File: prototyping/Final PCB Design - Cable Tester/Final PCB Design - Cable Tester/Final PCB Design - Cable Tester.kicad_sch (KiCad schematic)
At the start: 43 parts, among them J1 USB_B_Micro, J17 Banana Jack, J2 UPDI, J20 SFML-110-02-L-D-A, J4 MEM2061-01-188-00-A_REVA, J5 Barrel Jack 9V, J6 Touchscreen HMI, Q1 2N3904, SW1 Rocker Switch, U1 AVR128DB64x-xMR, U2 LP2985-3.3, U3 LM7805_TO220, U4 FT232RL, U6 J104D2C5VDC.15S, U7 CD74HC4050M96

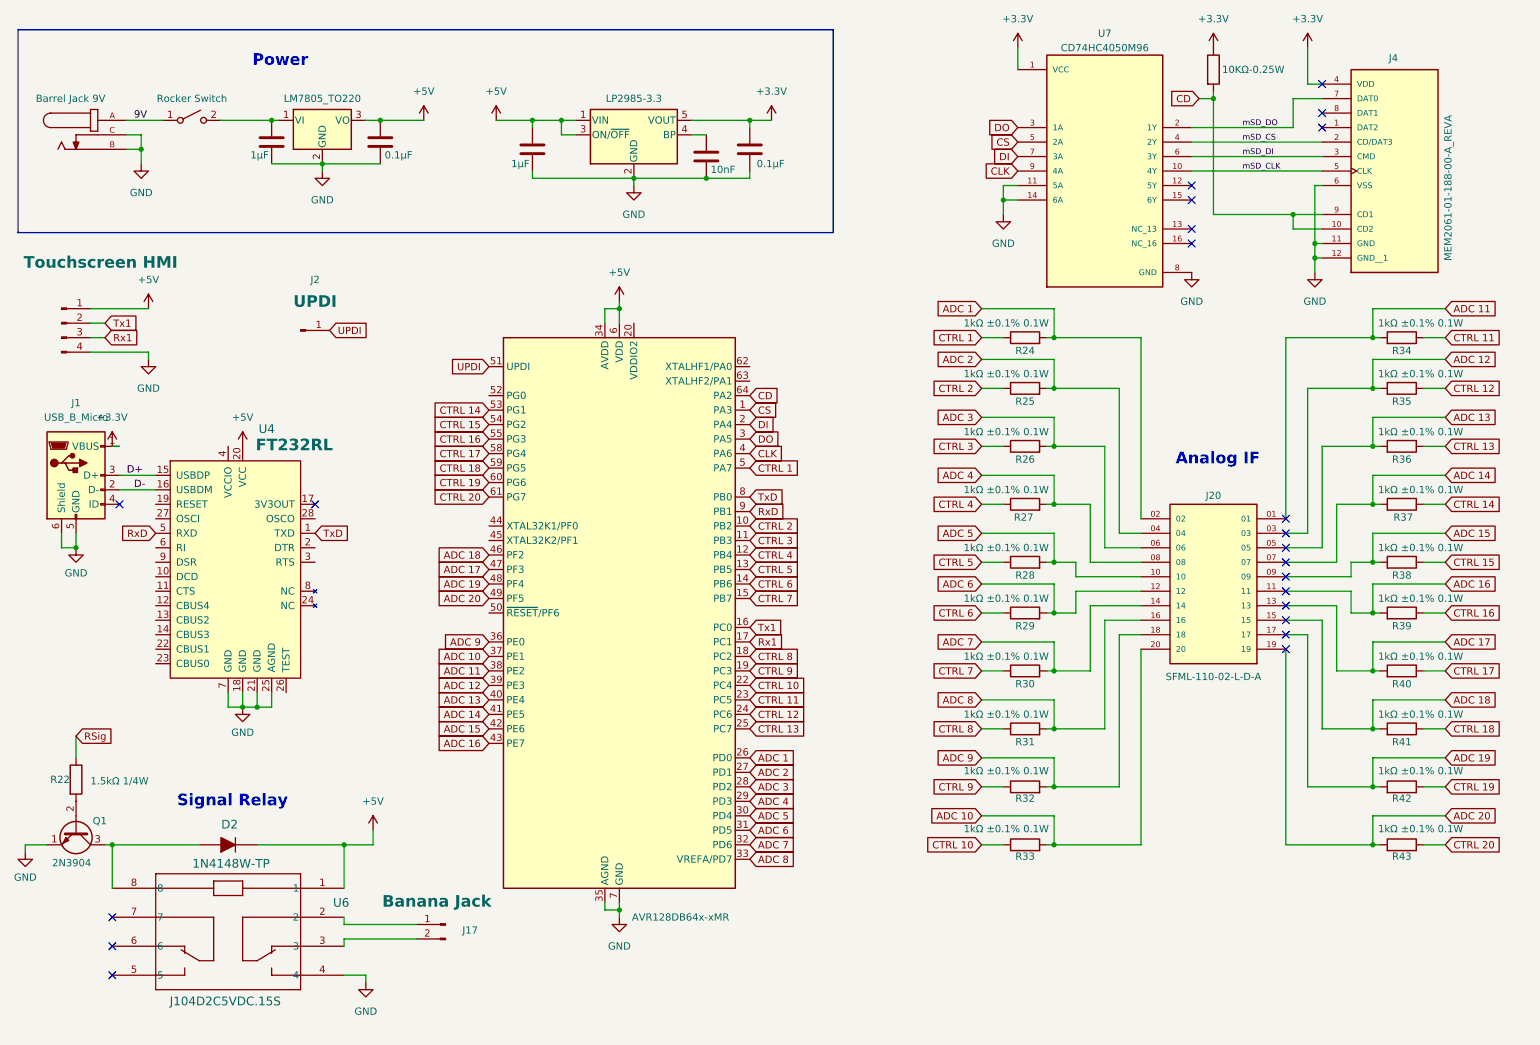
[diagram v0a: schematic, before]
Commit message: Final PCB Schematic and PCB layout update
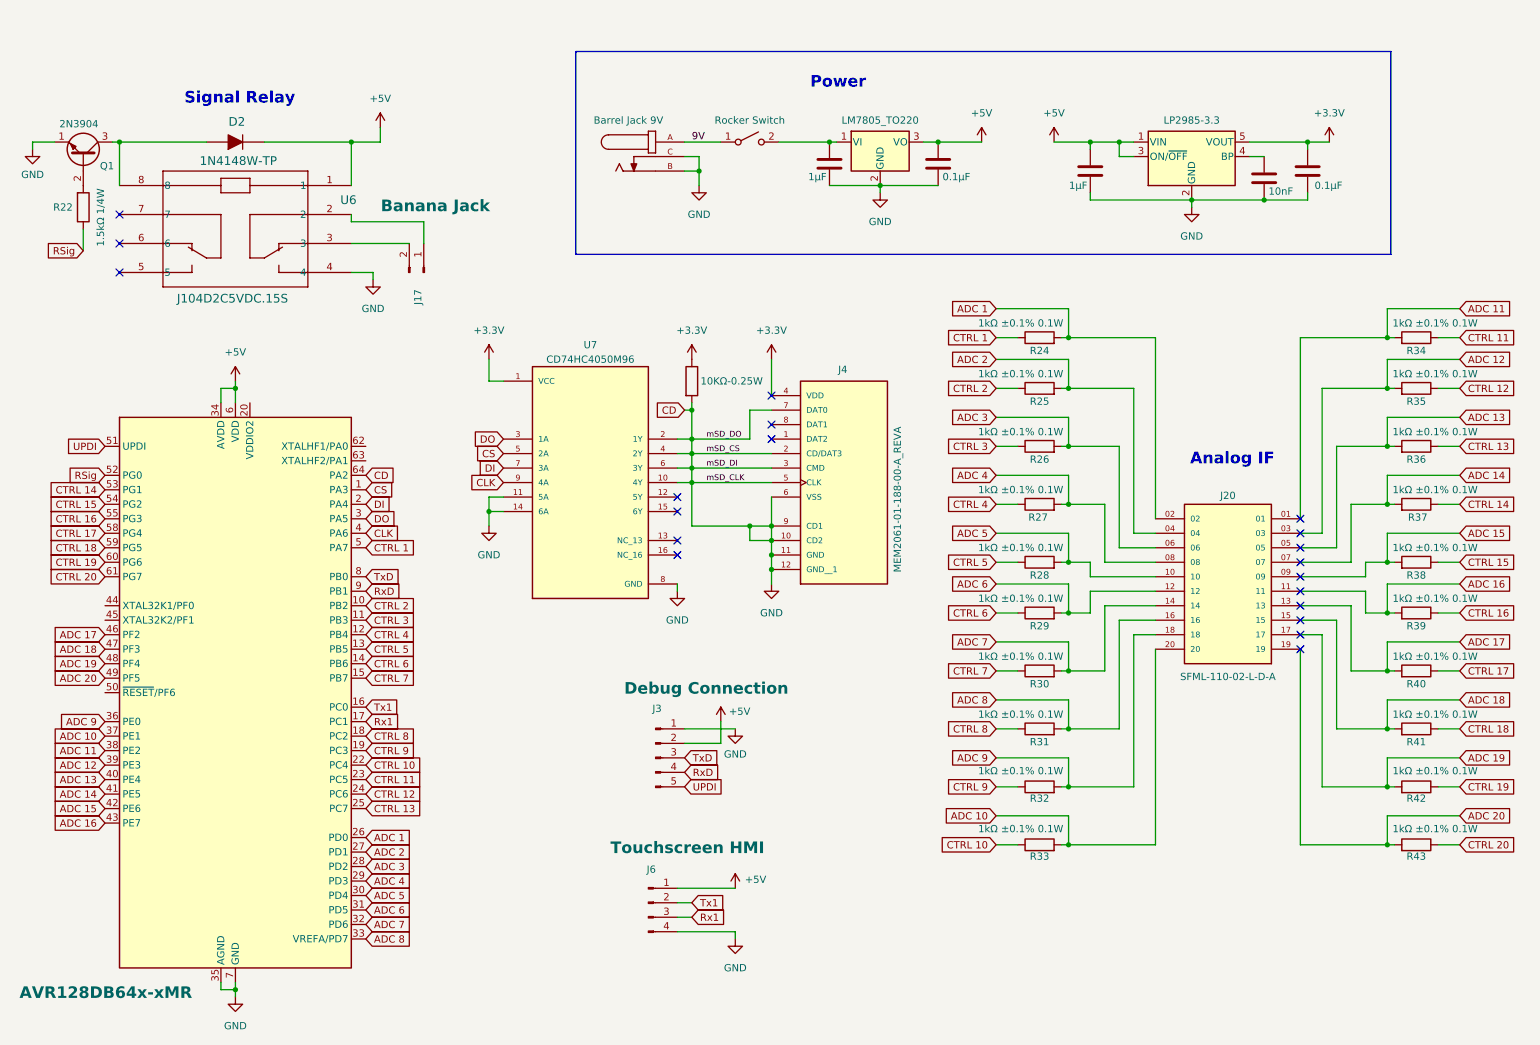
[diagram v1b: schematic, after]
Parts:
- removed J1: USB_B_Micro, Connector_USB:USB_Micro-AB_Molex_47590-0001, symbol Connector:USB_B_Micro
- removed J2: UPDI, Connector_PinHeader_2.54mm:PinHeader_1x01_P2.54mm_Vertical, symbol Connector:Conn_01x01_Pin
- removed U4: FT232RL, digikey-footprints:SSOP-28_W5.30mm, symbol dk_Interface-Controllers:FT232RL-REEL
- added J3: Debug Connection, Connector_PinHeader_2.54mm:PinHeader_1x05_P2.54mm_Vertical, symbol Connector:Conn_01x05_Pin
- SW1: footprint Connector_PinHeader_1.00mm:PinHeader_1x02_P1.00mm_Vertical -> Connector_PinHeader_2.54mm:PinHeader_1x02_P2.54mm_Vertical
- U7: footprint CD74HC4050M96:SOIC127P600X175-16N -> KiCad Symbols and Footprints:SOIC127P600X175-16N
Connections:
- net CD is gone; now on net GND: J4.10 (CD2), J4.9 (CD1), R2.2, U1.64 (PA2)
- net mSD_CLK is gone; now on net GND: J4.5 (CLK), U7.10 (4Y)
- net mSD_CS is gone; now on net GND: J4.2 (CD/DAT3), U7.4 (2Y)
- net mSD_DI is gone; now on net GND: J4.3 (CMD), U7.6 (3Y)
- net mSD_DO is gone; now on net GND: J4.7 (DAT0), U7.2 (1Y)
- net +5V: now also J3.2 (Pin_2)
- net ADC 17: now also U1.46 (PF2); no longer U1.47 (PF3)
- net ADC 18: now also U1.47 (PF3); no longer U1.46 (PF2)
- net GND: now also J3.1 (Pin_1)
- net RSig: now also U1.52 (PG0)
- net RxD: now also J3.4 (Pin_4)
- net TxD: now also J3.3 (Pin_3)
- net UPDI: now also J3.5 (Pin_5)
- no-connect marks 22 -> 20
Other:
- moved on the sheet: D2, J17, J20, J4, Q1, R22, R24, R25, R26, R27, R28, R29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
